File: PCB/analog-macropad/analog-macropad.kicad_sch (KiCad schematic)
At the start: 20 parts, among them U1 Teensy 4.1, U10 hall-effect sensor, U11 hall-effect sensor, U12 hall-effect sensor, U13 hall-effect sensor, U2 hall-effect sensor, U3 hall-effect sensor, U4 hall-effect sensor, U5 hall-effect sensor, U6 hall-effect sensor, U7 hall-effect sensor, U8 hall-effect sensor, U9 hall-effect sensor

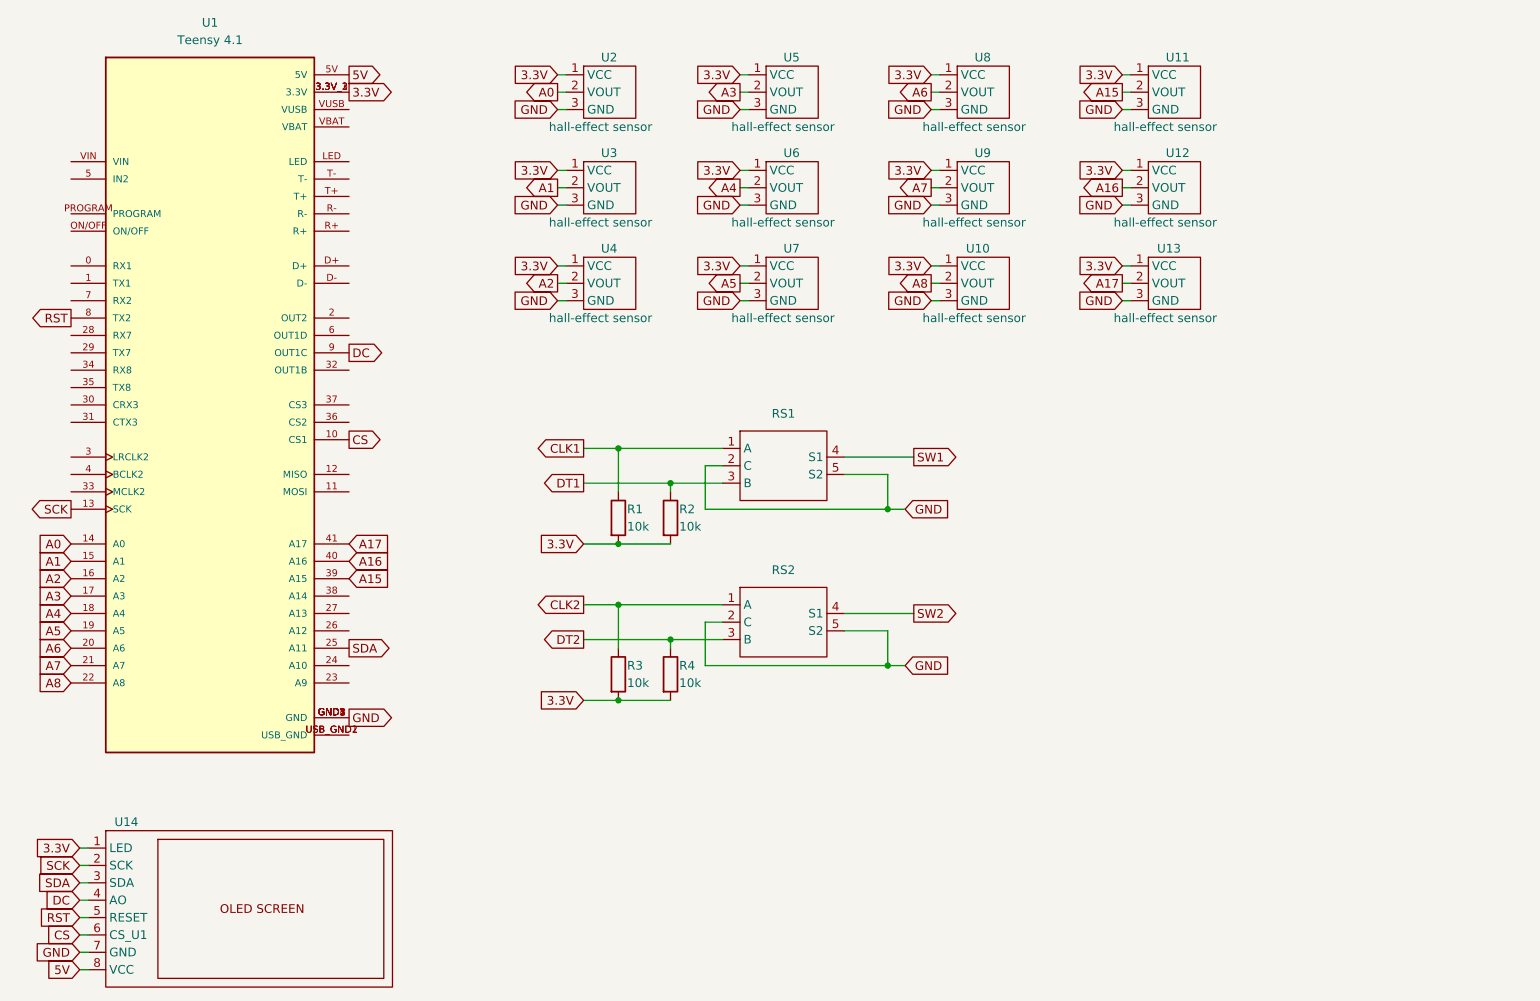
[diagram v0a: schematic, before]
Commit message: pcb finit pret a commander
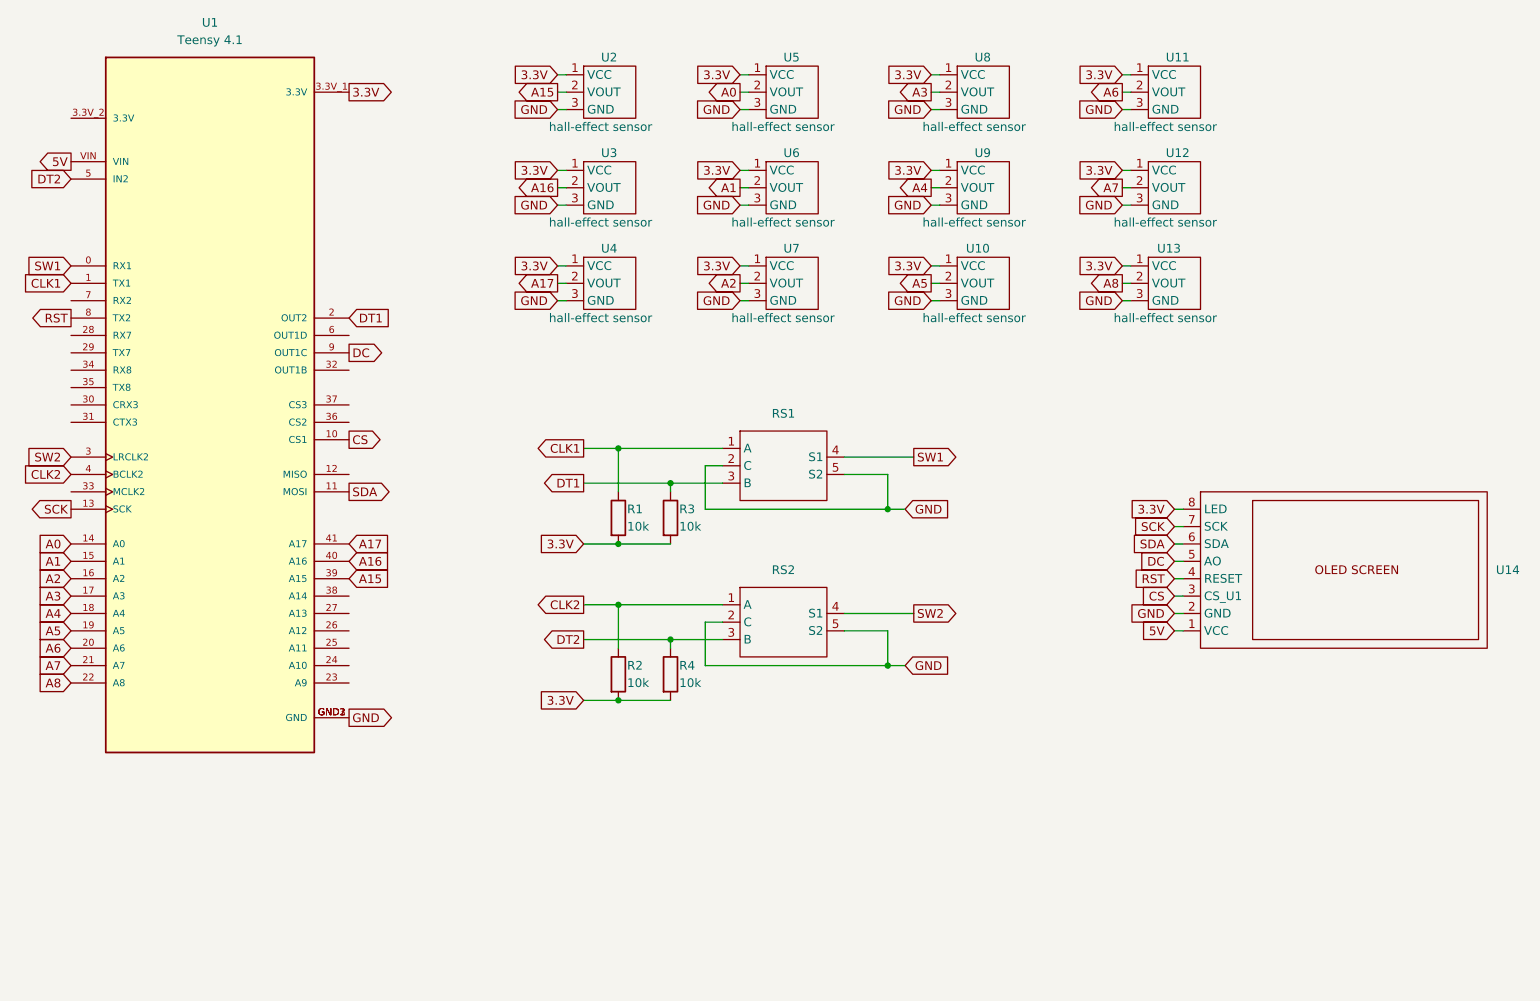
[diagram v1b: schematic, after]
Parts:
- R1, R4: footprint (none) -> Resistor_THT:R_Axial_DIN0207_L6.3mm_D2.5mm_P7.62mm_Horizontal
- R2: renamed from R3; footprint (none) -> Resistor_THT:R_Axial_DIN0207_L6.3mm_D2.5mm_P7.62mm_Horizontal
- R3: renamed from R2; footprint (none) -> Resistor_THT:R_Axial_DIN0207_L6.3mm_D2.5mm_P7.62mm_Horizontal
- RS1, RS2: footprint (none) -> analog-macropad:rotary encoder
- U10, U11, U12, U13, U2, U3, U4, U5, U6, U7, U8, U9: footprint (none) -> analog-macropad:hall sensor
- U14: footprint (none) -> analog-macropad:ST7735
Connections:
- net 3.3V: now also U14.8 (LED); no longer U1.3.3V_2 (3.3V), U1.3.3V_3 (3.3V), U14.1 (LED)
- net 5V: now also U1.VIN, U14.1 (VCC); no longer U1.5V, U14.8 (VCC)
- net A0: now also U5.2 (VOUT); no longer U2.2 (VOUT)
- net A1: now also U6.2 (VOUT); no longer U3.2 (VOUT)
- net A15: now also U2.2 (VOUT); no longer U11.2 (VOUT)
- net A16: now also U3.2 (VOUT); no longer U12.2 (VOUT)
- net A17: now also U4.2 (VOUT); no longer U13.2 (VOUT)
- net A2: now also U7.2 (VOUT); no longer U4.2 (VOUT)
- net A3: now also U8.2 (VOUT); no longer U5.2 (VOUT)
- net A4: now also U9.2 (VOUT); no longer U6.2 (VOUT)
- net A5: now also U10.2 (VOUT); no longer U7.2 (VOUT)
- net A6: now also U11.2 (VOUT); no longer U8.2 (VOUT)
- net A7: now also U12.2 (VOUT); no longer U9.2 (VOUT)
- net A8: now also U13.2 (VOUT); no longer U10.2 (VOUT)
- net CLK1: now also U1.1 (TX1)
- net CLK2: now also U1.4 (BCLK2)
- net CS: now also U14.3 (CS_U1); no longer U14.6 (CS_U1)
- net DC: now also U14.5 (AO); no longer U14.4 (AO)
- net DT1: now also U1.2 (OUT2)
- net DT2: now also U1.5 (IN2)
- net GND: now also U14.2 (GND); no longer U1.GND4 (GND), U1.GND5 (GND), U14.7 (GND)
- net RST: now also U14.4 (RESET); no longer U14.5 (RESET)
- net SCK: now also U14.7 (SCK); no longer U14.2 (SCK)
- net SDA: now also U1.11 (MOSI), U14.6 (SDA); no longer U1.25 (A11), U14.3 (SDA)
- net SW1: now also U1.0 (RX1)
- net SW2: now also U1.3 (LRCLK2)
